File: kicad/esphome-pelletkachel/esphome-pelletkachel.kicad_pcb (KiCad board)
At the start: 2 copper layers, 38.1 x 76.2 mm, 13 parts, among them J6 1-wire, U1 ESP32-DEVKITC-32U, U2 757

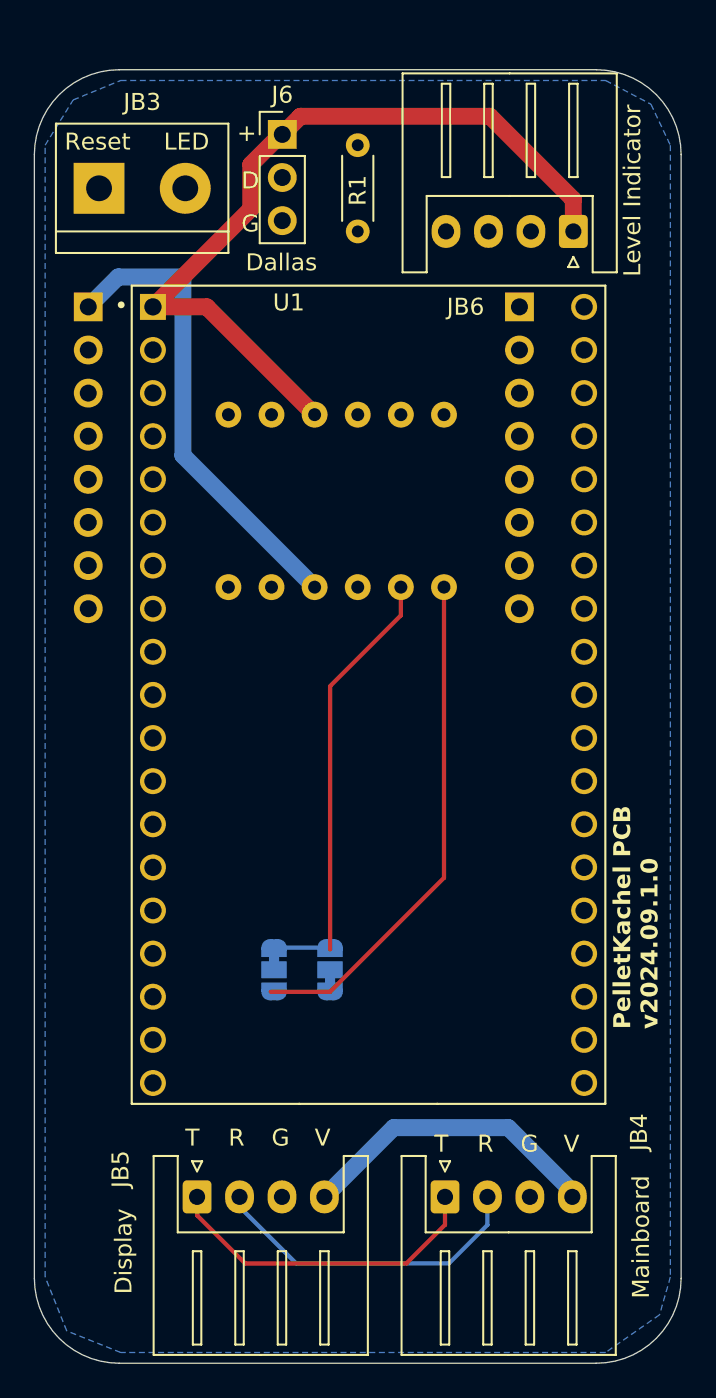
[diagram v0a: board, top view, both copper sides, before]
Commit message: autorouted
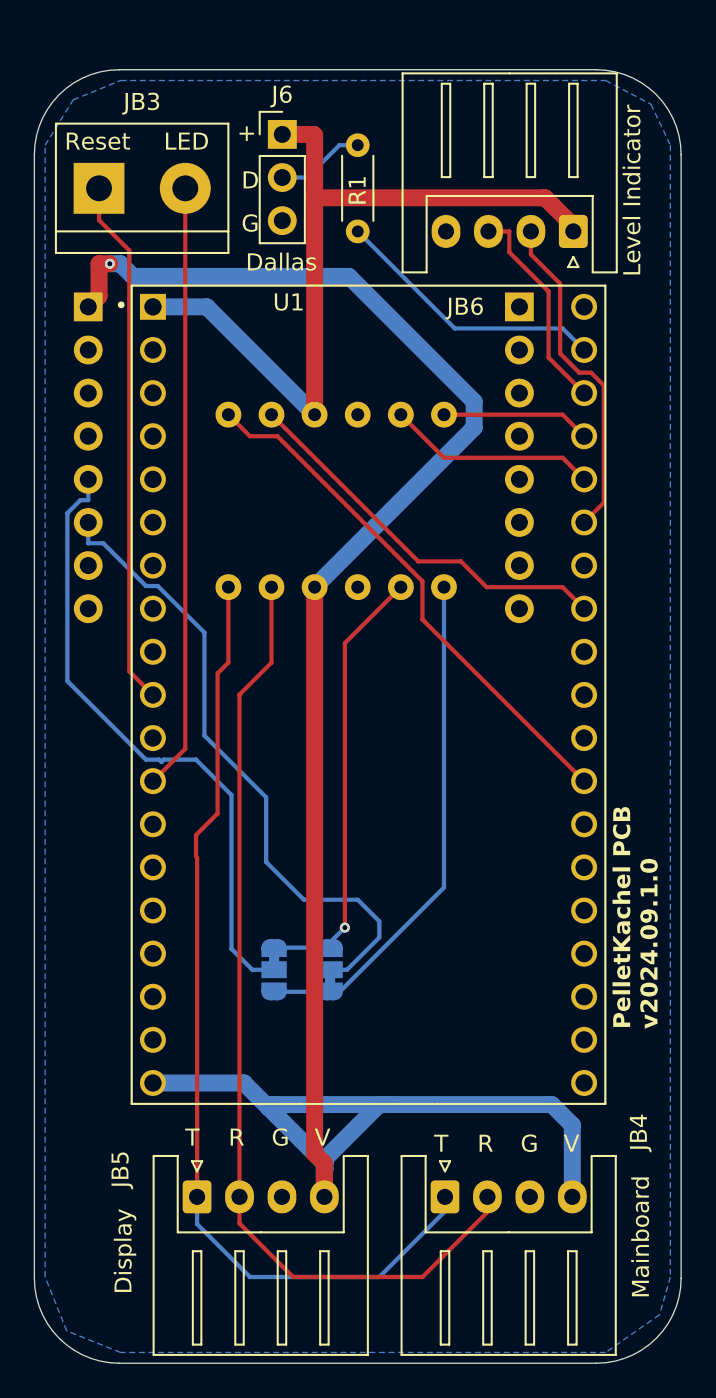
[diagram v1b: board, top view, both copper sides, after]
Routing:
- net +5V: track 46.0 -> 123.6 mm, vias 0 -> 1
- net /TX to Display (HV): track 0.00 -> 38.0 mm
- net /MCURX: track 19.2 -> 56.7 mm
- net /RX to Display (HV): track 0.00 -> 37.3 mm
- net /MCUTX: track 19.5 -> 56.7 mm
- net /LED: track 0.00 -> 35.7 mm
- net /MCU UART TX Read: track 0.00 -> 31.2 mm
- net /Reset: track 0.00 -> 31.2 mm
- net /MCU UART RX Read: track 0.00 -> 23.1 mm
- net /SDA: track 0.00 -> 19.8 mm
- net Net-(U1-IO23): track 0.00 -> 16.2 mm
- net /SCL: track 0.00 -> 12.6 mm
- net /RX to Display: track 0.00 -> 12.4 mm
- net /TX to Display: track 0.00 -> 8.78 mm
- net Net-(J6-Pin_2): track 0.00 -> 5.23 mm
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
